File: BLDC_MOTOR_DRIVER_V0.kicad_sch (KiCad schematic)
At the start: 17 parts, among them Q1 N-MOSFET, Q2 N-MOSFET, Q3 N-MOSFET, Q4 N-MOSFET, Q5 N-MOSFET, Q6 N-MOSFET, U1 3-phase Gate Driver, U2 Micro controller

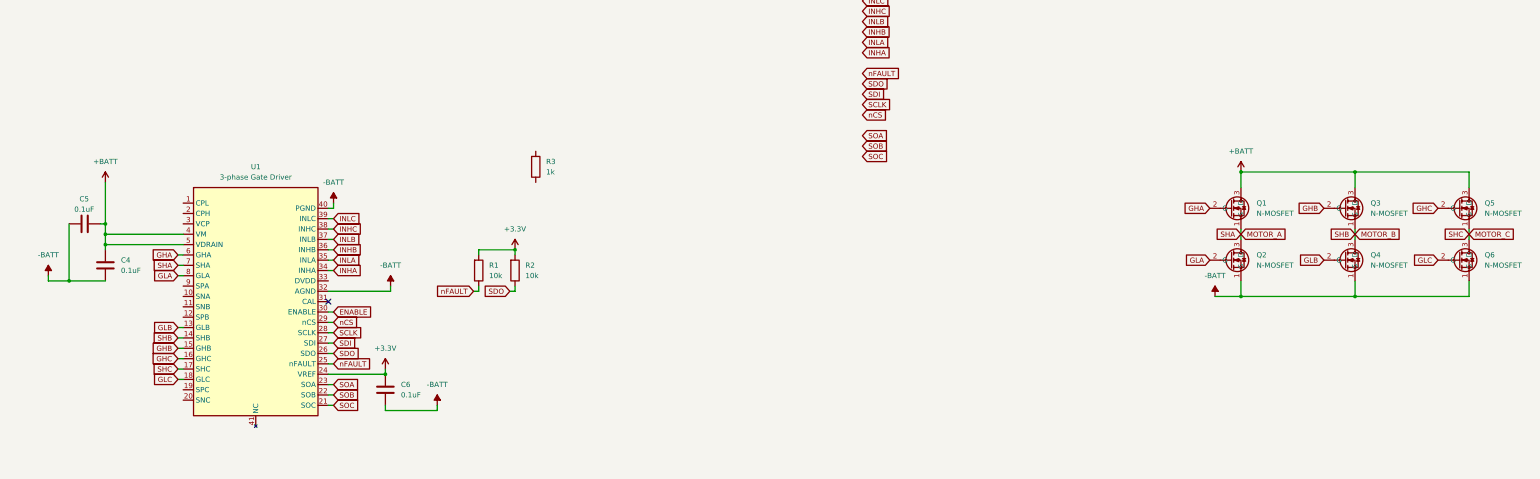
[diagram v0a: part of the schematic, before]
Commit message: update
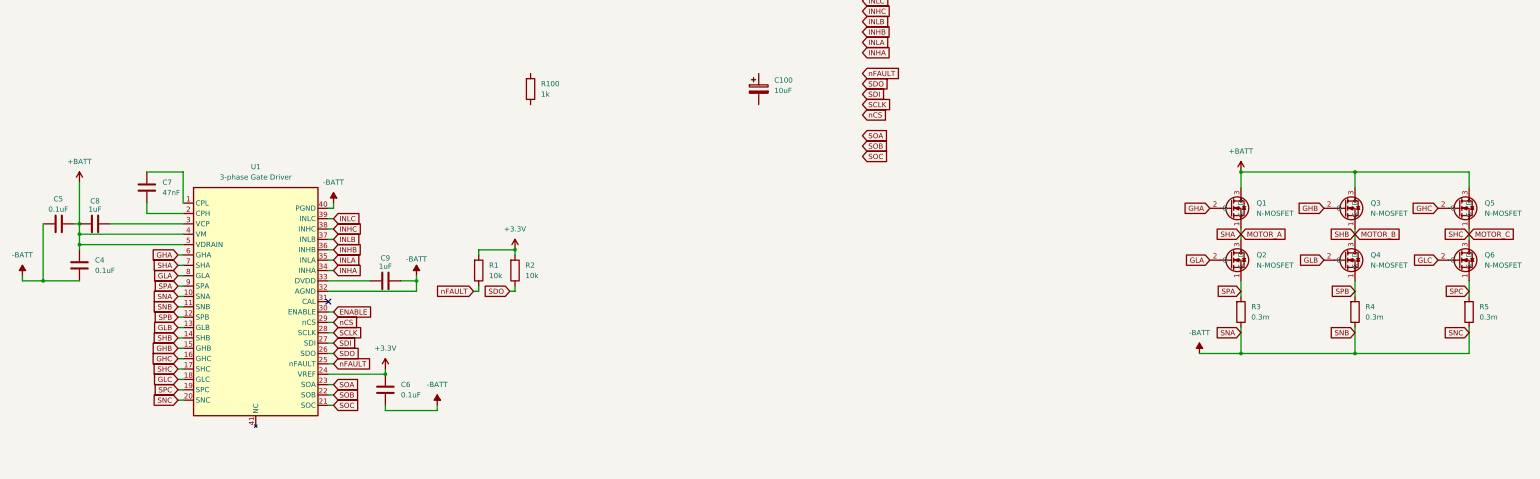
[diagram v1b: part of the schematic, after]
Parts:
- added C100: 10uF, Capacitor_SMD:C_Elec_5x5.4, symbol EMK1VM100D80D00R:EMK1VM100D80D00R
- added C7: 47nF, Capacitor_SMD:C_0402_1005Metric, symbol CGA2B3X7R1H473K050BB:CGA2B3X7R1H473K050BB
- added C8, C9: 1uF, Capacitor_SMD:C_0805_2012Metric, symbol CL21B105KBFNNNE:CL21B105KBFNNNE
- added R3, R4, R5: 0.3m, Resistor_SMD:R_2512_6332Metric, symbol CSNL2512FTL300:CSNL2512FTL300
- renumbered R3 to R100
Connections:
- net +BATT: now also C8.1
- net -BATT: now also U1.10 (SNA), U1.11 (SNB), U1.20 (SNC), C9.2, R3.2, R4.2, R5.2; no longer Q2.1 (S), Q4.1 (S), Q6.1 (S)
- net at U1.1 (CPL): now also C7.1
- net SPB: now reaches U1.12 (SPB)
- net SPB: now also Q4.1 (S), R4.1
- net SPC: now reaches U1.19 (SPC)
- net SPC: now also Q6.1 (S), R5.1
- net at U1.2 (CPH): now also C7.2
- net at U1.3 (VCP): now also C8.2
- net at U1.33 (DVDD): now also C9.1
- net SPA: now reaches U1.9 (SPA)
- net SPA: now also Q2.1 (S), R3.1
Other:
- moved on the sheet: C4, C5, R100

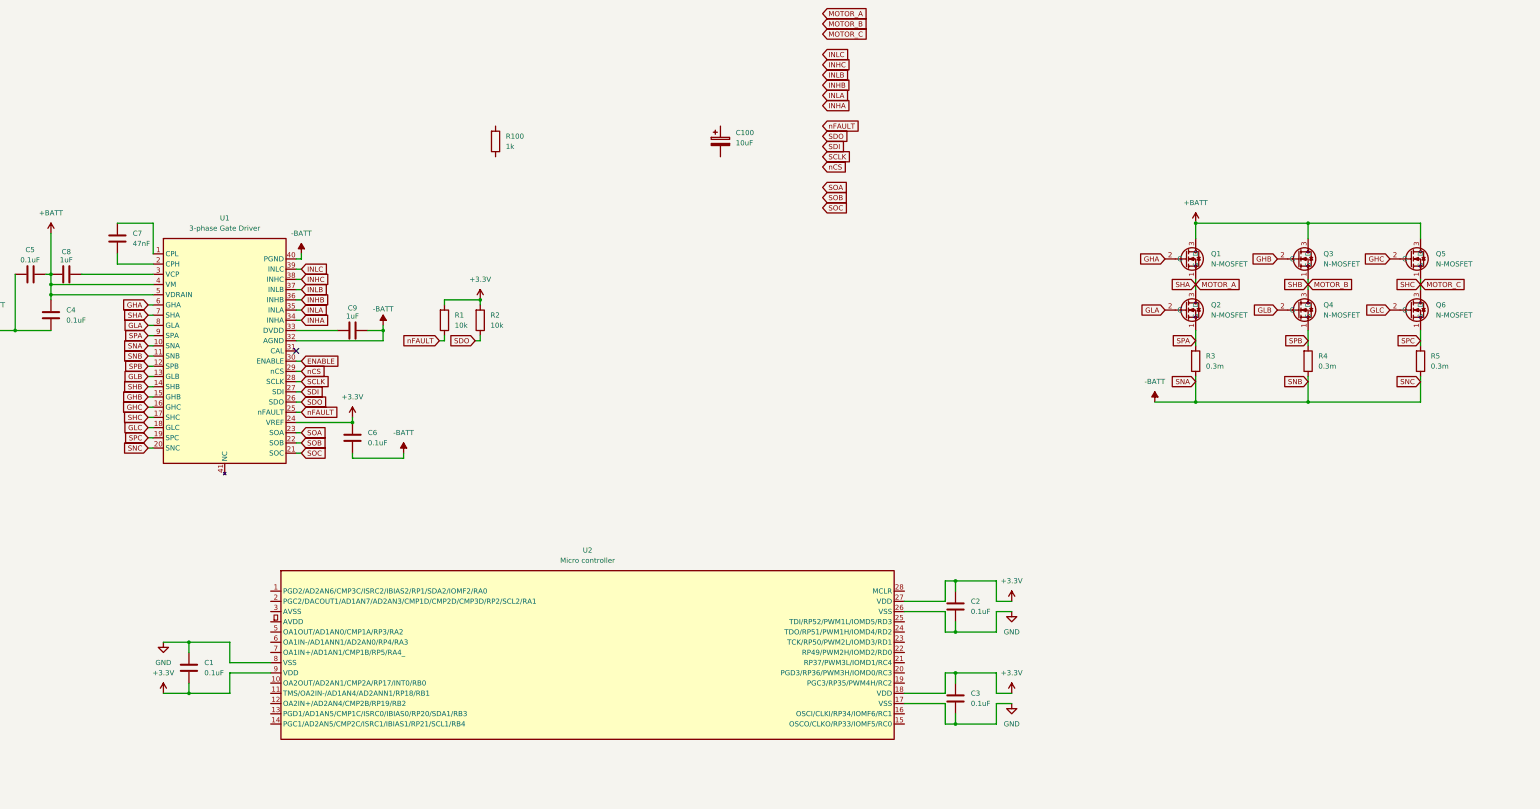
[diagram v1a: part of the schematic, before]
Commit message: dftg
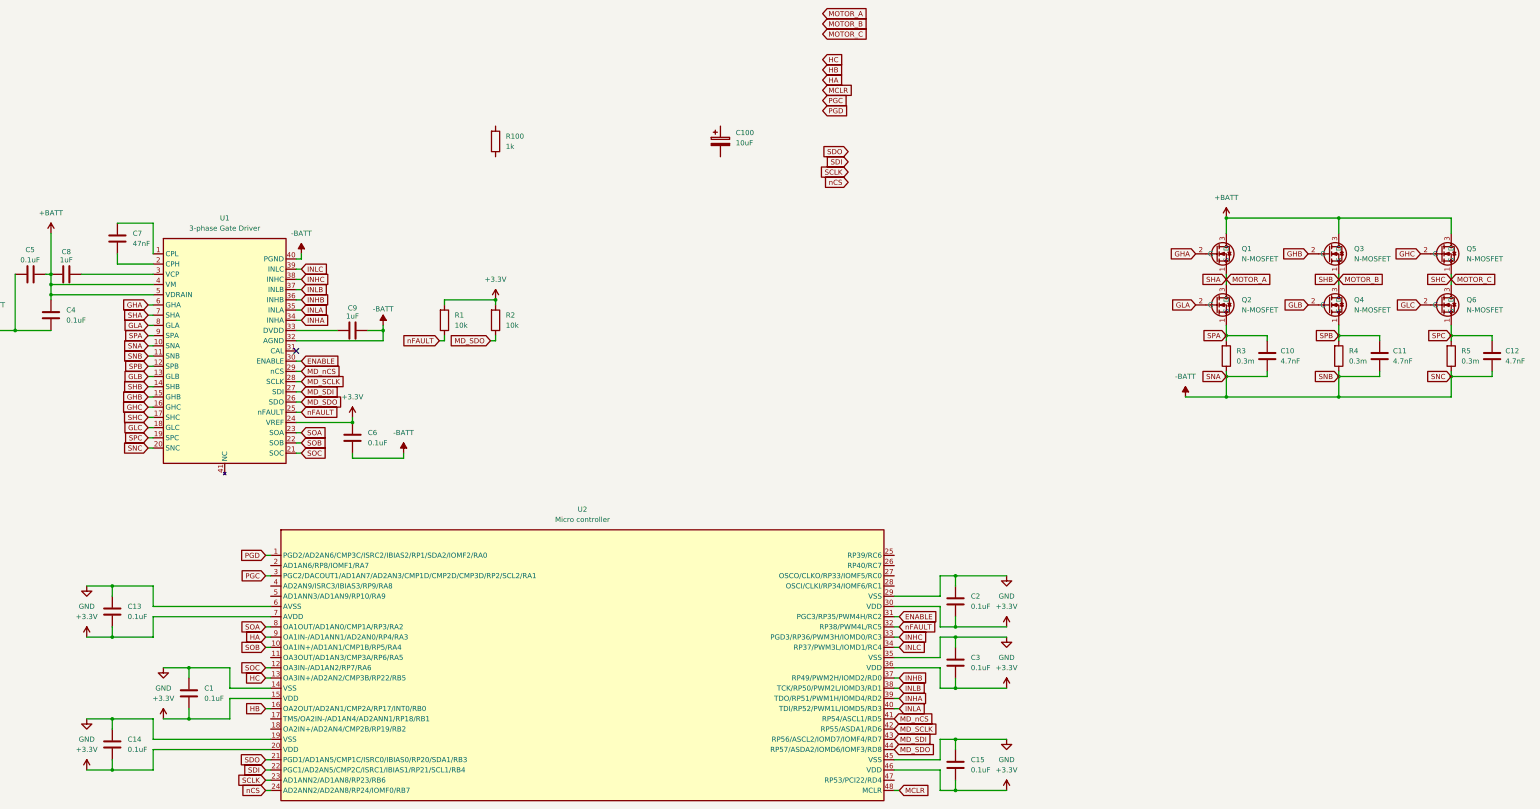
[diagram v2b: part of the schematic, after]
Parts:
- removed U2: Micro controller, Package_SO:SSOP-28_5.3x10.2mm_P0.65mm, symbol DSPIC33AK32MC102:DSPIC33AK32MC102
- added C10, C11, C12: 4.7nF, Capacitor_SMD:C_0603_1608Metric, symbol CC0603KRX7R9BB472:CC0603KRX7R9BB472
- added C13, C14, C15: 0.1uF, Capacitor_SMD:C_0603_1608Metric, symbol GRM188F11H104ZA01:GRM188F11H104ZA01
- added U2: Micro controller, Package_QFP:TQFP-48_7x7mm_P0.5mm, symbol DSPIC33AK32MC105:DSPIC33AK32MC105
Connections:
- net +3.3V: now also C2.2, C3.2, C13.2, C14.2, C15.2, U2.15 (VDD), U2.20 (VDD), U2.30 (VDD), U2.36 (VDD), U2.46 (VDD), U2.7 (AVDD); no longer C2.1, C3.1
- net -BATT: now also C10.2, C11.2, C12.2
- net ENABLE: now also U2.31 (PGC3/RP35/PWM4H/RC2)
- net GND: now also C2.1, C3.1, C13.1, C14.1, C15.1, U2.14 (VSS), U2.19 (VSS), U2.29 (VSS), U2.35 (VSS), U2.45 (VSS), U2.6 (AVSS); no longer C2.2, C3.2
- net INHA: now also U2.39 (TDO/RP51/PWM1H/IOMD4/RD2)
- net INHB: now also U2.37 (RP49/PWM2H/IOMD2/RD0)
- net INHC: now also U2.33 (PGD3/RP36/PWM3H/IOMD0/RC3)
- net INLA: now also U2.40 (TDI/RP52/PWM1L/IOMD5/RD3)
- net INLB: now also U2.38 (TCK/RP50/PWM2L/IOMD3/RD1)
- net INLC: now also U2.34 (RP37/PWM3L/IOMD1/RC4)
- net SCLK: now also U2.23 (AD1ANN2/AD1AN8/RP23/RB6); no longer U1.28 (SCLK)
- net SDI: now also U2.22 (PGC1/AD2AN5/CMP2C/ISRC1/IBIAS1/RP21/SCL1/RB4); no longer U1.27 (SDI)
- net SDO: now also U2.21 (PGD1/AD1AN5/CMP1C/ISRC0/IBIAS0/RP20/SDA1/RB3); no longer R2.2, U1.26 (SDO)
- net SOA: now also U2.8 (OA1OUT/AD1AN0/CMP1A/RP3/RA2)
- net SOB: now also U2.10 (OA1IN+/AD1AN1/CMP1B/RP5/RA4)
- net SOC: now also U2.12 (OA3IN-/AD1AN2/RP7/RA6)
- net SPA: now also C10.1
- net SPB: now also C11.1
- net SPC: now also C12.1
- net nCS: now also U2.24 (AD2ANN2/AD2AN8/RP24/IOMF0/RB7); no longer U1.29 (nCS)
- net nFAULT: now also U2.32 (RP38/PWM4L/RC5)
- new net HA: U2.9 (OA1IN-/AD1ANN1/AD2AN0/RP4/RA3)
- new net HB: U2.16 (OA2OUT/AD2AN1/CMP2A/RP17/INT0/RB0)
- new net HC: U2.13 (OA3IN+/AD2AN2/CMP3B/RP22/RB5)
- new net MCLR: U2.48 (MCLR)
- new net MD_SCLK: U1.28 (SCLK), U2.42 (RP55/ASDA1/RD6)
- new net MD_SDI: U1.27 (SDI), U2.43 (RP56/ASCL2/IOMD7/IOMF4/RD7)
- new net MD_SDO: R2.2, U1.26 (SDO), U2.44 (RP57/ASDA2/IOMD6/IOMF3/RD8)
- new net MD_nCS: U1.29 (nCS), U2.41 (RP54/ASCL1/RD5)
- new net PGC: U2.3 (PGC2/DACOUT1/AD1AN7/AD2AN3/CMP1D/CMP2D/CMP3D/RP2/SCL2/RA1)
- new net PGD: U2.1 (PGD2/AD2AN6/CMP3C/ISRC2/IBIAS2/RP1/SDA2/IOMF2/RA0)
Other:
- moved on the sheet: C1, C2, Q1, Q2, Q3, Q4, Q5, Q6, R2, R3, R4, R5

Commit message: update
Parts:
- removed C100: 10uF, Capacitor_SMD:C_Elec_5x5.4, symbol EMK1VM100D80D00R:EMK1VM100D80D00R
- removed R100: 1k, Resistor_SMD:R_0603_1608Metric, symbol NRC06F1001TRF:NRC06F1001TRF
- added C16, C18, C19, C20: 10uF, Capacitor_SMD:C_Elec_5x5.4, symbol EMK1VM100D80D00R:EMK1VM100D80D00R
- added C17, C21, C22: 0.1uF, Capacitor_SMD:C_0603_1608Metric, symbol GRM188F11H104ZA01:GRM188F11H104ZA01
- added J1: Conn_01x05_Pin, Connector_PinHeader_2.54mm:PinHeader_1x05_P2.54mm_Vertical, symbol Connector:Conn_01x05_Pin
- added J10, J7, J8, J9: Conn_01x01_Socket, Connector_Wire:SolderWirePad_1x01_SMD_2x4mm, symbol Connector:Conn_01x01_Socket
- added J2, J3, J4, J5, J6: Conn_01x01_Socket, Connector_Wire:SolderWirePad_1x01_SMD_3x6mm, symbol Connector:Conn_01x01_Socket
- added R6: 10k, Resistor_SMD:R_0603_1608Metric, symbol NRC06F1002TRF:NRC06F1002TRF
- added U3: 3.3V Regurator, Package_TO_SOT_SMD:SOT-89-3, symbol SL7333-8:SL7333-8
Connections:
- net GND is gone; now on net -BATT: C1.1, C13.1, C14.1, C15.1, C2.1, C3.1, U2.14 (VSS), U2.19 (VSS), U2.29 (VSS), U2.35 (VSS), U2.45 (VSS), U2.6 (AVSS)
- net +3.3V: now also C19.1, J1.2 (Pin_2), R6.2, U3.3 (VOUT)
- net +BATT: now also C16.1, C17.1, C20.1, C21.1, C22.1, J2.1 (Pin_1)
- net -BATT: now also C16.2, C17.2, C18.2, C19.2, C20.2, C21.2, C22.2, J1.3 (Pin_3), J3.1 (Pin_1), U3.1 (GND)
- net HA: now also J10.1 (Pin_1)
- net HB: now also J9.1 (Pin_1)
- net HC: now also J8.1 (Pin_1)
- net MCLR: now also J1.1 (Pin_1), R6.1
- net MOTOR_A: now also J4.1 (Pin_1)
- net MOTOR_B: now also J5.1 (Pin_1)
- net MOTOR_C: now also J6.1 (Pin_1)
- net PGC: now also J1.5 (Pin_5)
- net PGD: now also J1.4 (Pin_4)
- net SCLK: no longer names the net of U2.23 (AD1ANN2/AD1AN8/RP23/RB6)
- net SDI: no longer names the net of U2.22 (PGC1/AD2AN5/CMP2C/ISRC1/IBIAS1/RP21/SCL1/RB4)
- net SDO: no longer names the net of U2.21 (PGD1/AD1AN5/CMP1C/ISRC0/IBIAS0/RP20/SDA1/RB3)
- net nCS: no longer names the net of U2.24 (AD2ANN2/AD2AN8/RP24/IOMF0/RB7)
- new net VDC: C18.1, J7.1 (Pin_1), U3.2 (VIN)
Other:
- moved on the sheet: C1, C10, C11, C12, C13, C14, C15, C2, C3, C4, C5, C6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

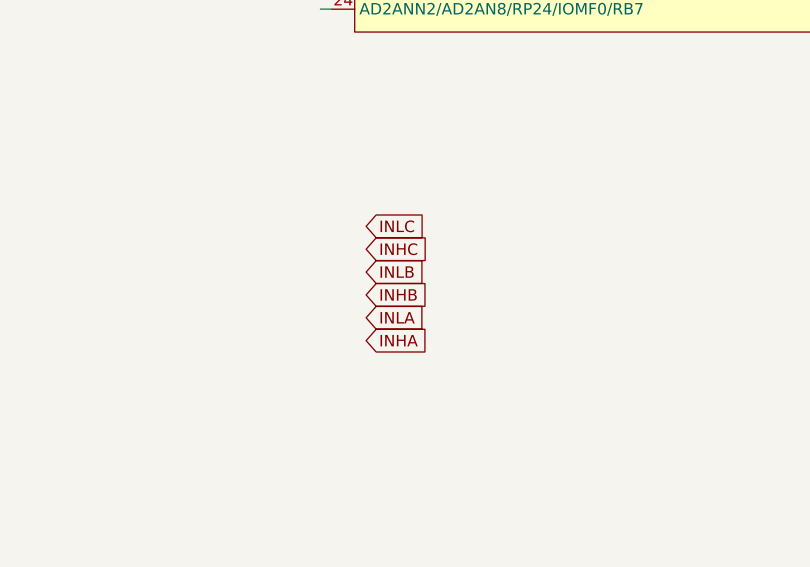
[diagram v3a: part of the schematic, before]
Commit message: update
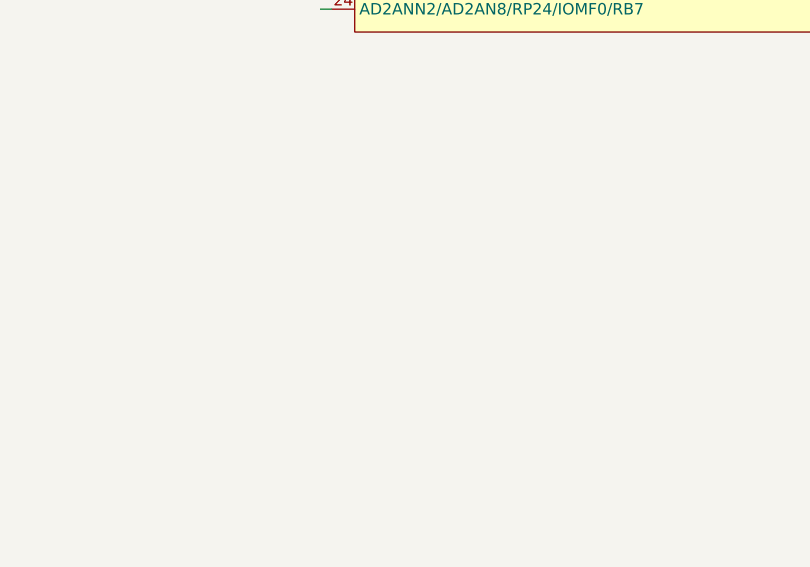
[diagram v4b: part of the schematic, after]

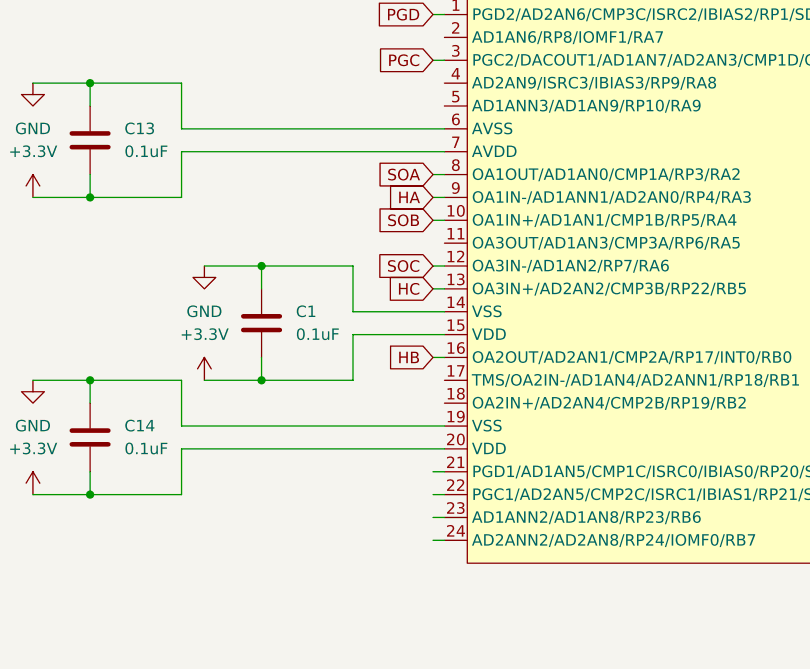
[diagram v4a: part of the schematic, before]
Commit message: upda
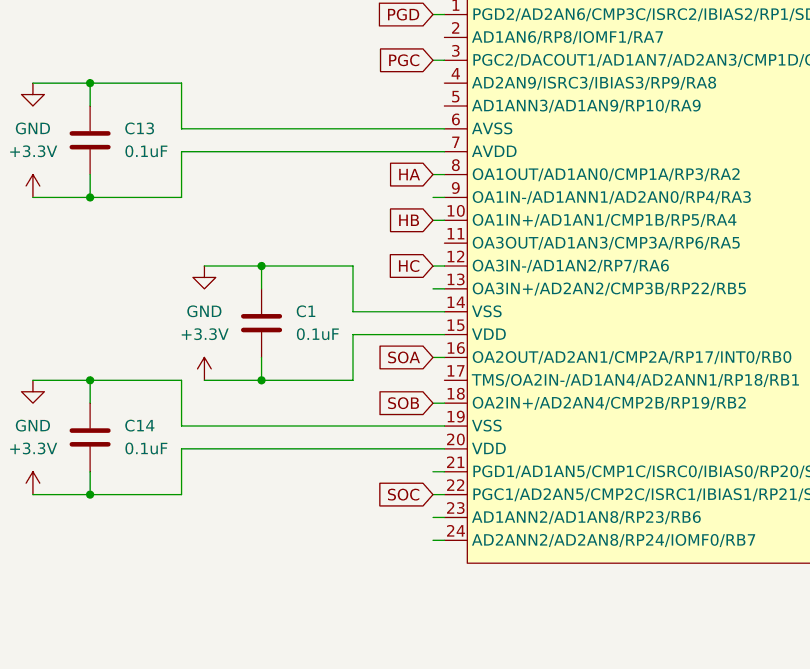
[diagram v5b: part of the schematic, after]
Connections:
- net HA: now also U2.8 (OA1OUT/AD1AN0/CMP1A/RP3/RA2); no longer U2.9 (OA1IN-/AD1ANN1/AD2AN0/RP4/RA3)
- net HB: now also U2.10 (OA1IN+/AD1AN1/CMP1B/RP5/RA4); no longer U2.16 (OA2OUT/AD2AN1/CMP2A/RP17/INT0/RB0)
- net HC: now also U2.12 (OA3IN-/AD1AN2/RP7/RA6); no longer U2.13 (OA3IN+/AD2AN2/CMP3B/RP22/RB5)
- net SOA: now also U2.16 (OA2OUT/AD2AN1/CMP2A/RP17/INT0/RB0); no longer U2.8 (OA1OUT/AD1AN0/CMP1A/RP3/RA2)
- net SOB: now also U2.18 (OA2IN+/AD2AN4/CMP2B/RP19/RB2); no longer U2.10 (OA1IN+/AD1AN1/CMP1B/RP5/RA4)
- net SOC: now also U2.22 (PGC1/AD2AN5/CMP2C/ISRC1/IBIAS1/RP21/SCL1/RB4); no longer U2.12 (OA3IN-/AD1AN2/RP7/RA6)
